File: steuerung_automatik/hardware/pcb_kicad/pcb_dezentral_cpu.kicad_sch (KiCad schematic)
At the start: 35 parts, among them J1 USB_C_Receptacle_USB2.0, SW2 SW_MEC_5E, U1 RP2040, U3 W25Q128JVS, U4 AMS1117-3.3, Y1 Crystal_GND24_Small

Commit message: pcb_dezentral, update J1/J2, v0.8
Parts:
- IO18, IO19, IO20: now left out of the parts list
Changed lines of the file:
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@@
   )
   (symbol (lib_id "Connector:TestPoint") (at 41.148 95.504 90) (unit 1)
-    (in_bom yes) (on_board yes) (dnp no)
+    (in_bom no) (on_board yes) (dnp no)
     (property "Reference" "IO19" (at 34.798 95.504 90)
       (effects (font (size 1.27 1.27)))
@@
   )
   (symbol (lib_id "Connector:TestPoint") (at 41.148 92.964 90) (unit 1)
-    (in_bom yes) (on_board yes) (dnp no)
+    (in_bom no) (on_board yes) (dnp no)
     (property "Reference" "IO18" (at 34.798 92.964 90)
       (effects (font (size 1.27 1.27)))
@@
   )
   (symbol (lib_id "Connector:TestPoint") (at 41.148 98.044 90) (unit 1)
-    (in_bom yes) (on_board yes) (dnp no)
+    (in_bom no) (on_board yes) (dnp no)
     (property "Reference" "IO20" (at 34.798 98.044 90)
       (effects (font (size 1.27 1.27)))

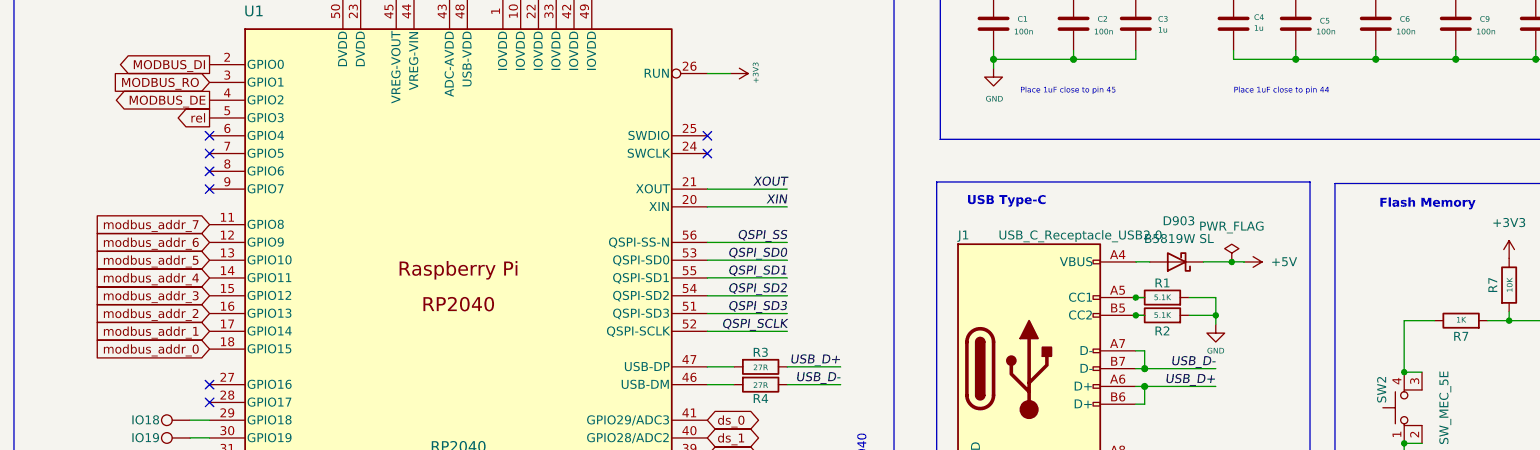
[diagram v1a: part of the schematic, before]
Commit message: pcb_dezentral v1.0
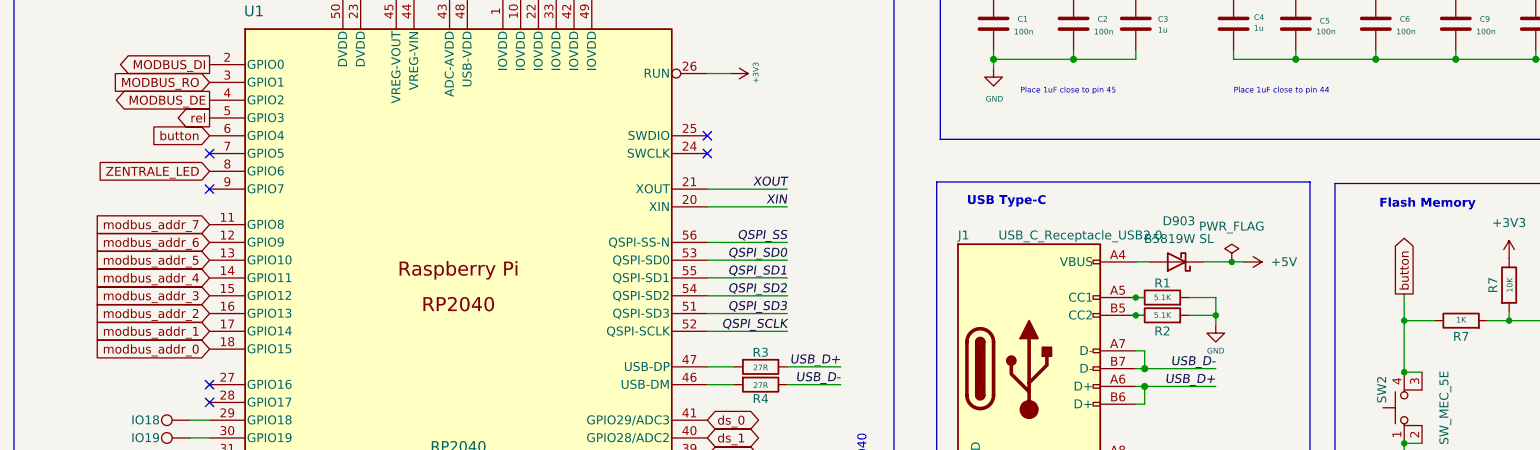
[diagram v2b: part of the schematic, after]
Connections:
- net button: now reaches R7.1, SW2.3 (K), SW2.4 (A)
- net button: now also U1.6 (GPIO4)
- net ZENTRALE_LED: now reaches U1.8 (GPIO6)
- no-connect marks 11 -> 9
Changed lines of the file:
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@@
   (junction (at 262.128 69.85) (diameter 0) (color 0 0 0 0)
   )
+  (junction (at 214.63 78.74) (diameter 0) (color 0 0 0 0)
+  )
   (junction (at 79.502 120.904) (diameter 1.016) (color 0 0 0 0)
   )
@@
   )
   (no_connect (at 176.276 100.838))
-  (no_connect (at 43.942 52.324))
   (no_connect (at 176.276 98.298))
   (no_connect (at 115.062 52.324))
@@
   (no_connect (at 43.942 54.864))
   (no_connect (at 43.942 59.944))
-  (no_connect (at 43.942 57.404))
   (wire (pts (xy 98.552 32.004) (xy 98.552 29.464))
     (stroke (width 0) (type solid))
@@
   )
   (wire (pts (xy 244.348 141.732) (xy 244.348 144.272))
+    (stroke (width 0) (type default))
+  )
+  (wire (pts (xy 214.63 74.93) (xy 214.63 78.74))
     (stroke (width 0) (type default))
   )
@@
     )
   )
+  (global_label "ZENTRALE_LED" (shape input) (at 43.942 57.404 180) (fields_autoplaced)
+    (effects (font (size 1.27 1.27)) (justify right))
+    (property "Intersheetrefs" "${INTERSHEET_REFS}" (at 27.2547 57.404 0)
+      (effects (font (size 1.27 1.27)) (justify right) hide)
+    )
+  )
   (global_label "MODBUS_DE" (shape output) (at 43.942 47.244 180) (fields_autoplaced)
     (effects (font (size 1.27 1.27)) (justify right))
@@
     )
   )
+  (global_label "button" (shape output) (at 214.63 74.93 90) (fields_autoplaced)
+    (effects (font (size 1.27 1.27)) (justify left))
+    (property "Intersheetrefs" "${INTERSHEET_REFS}" (at 214.63 65.8023 90)
+      (effects (font (size 1.27 1.27)) (justify left) hide)
+    )
+  )
   (global_label "ds_7" (shape bidirectional) (at 43.942 103.124 180) (fields_autoplaced)
     (effects (font (size 1.27 1.27)) (justify right))
@@
       (effects (font (size 1.27 1.27)) (justify right) hide)
     )
+  )
+  (global_label "button" (shape input) (at 43.942 52.324 180) (fields_autoplaced)
+    (effects (font (size 1.27 1.27)) (justify right))
+    (property "Intersheetrefs" "${INTERSHEET_REFS}" (at 34.8143 52.324 0)
+      (effects (font (size 1.27 1.27)) (justify right) hide)
+    )
